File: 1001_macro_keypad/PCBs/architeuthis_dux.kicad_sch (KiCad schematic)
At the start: 32 parts, among them J1 ePaperModule, J2 RotaryModule_01, J3 RotaryModule_02, SW01 MX_SW, SW10 MX_SW, SW11 MX_SW, SW12 MX_SW, SW13 MX_SW, SW14 MX_SW, SW2 MX_SW, SW3 MX_SW, SW4 MX_SW, SW5 MX_SW, SW6 MX_SW, SW7 MX_SW, SW8 MX_SW, SW9 MX_SW, U1 Pico

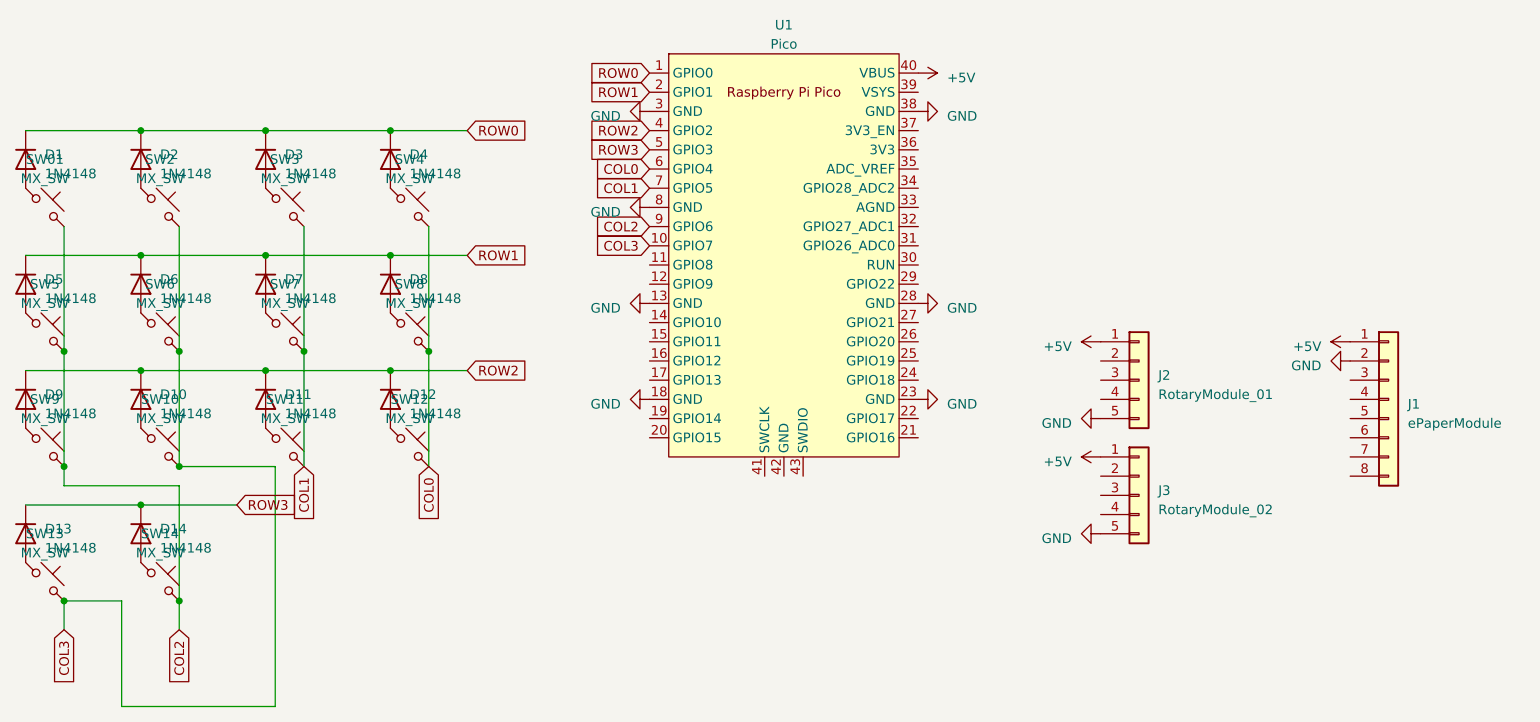
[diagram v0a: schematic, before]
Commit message: 배선작업 거의 완료
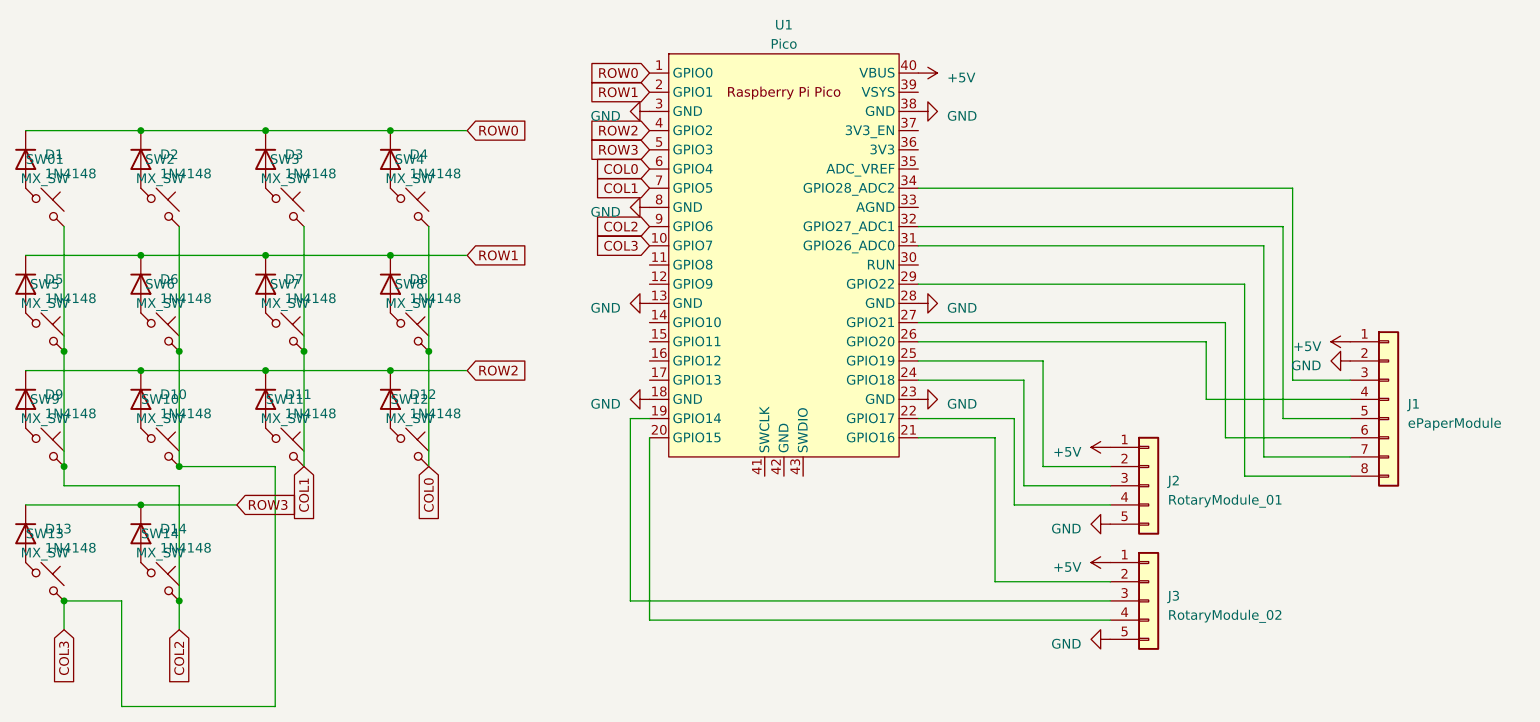
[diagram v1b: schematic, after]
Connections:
- net at J1.3 (D/C): now also U1.34 (GPIO28_ADC2)
- net at J1.4 (CS): now also U1.26 (GPIO20)
- net at J1.5 (SCL): now also U1.32 (GPIO27_ADC1)
- net at J1.6 (SDA): now also U1.27 (GPIO21)
- net at J1.7 (GND): now also U1.31 (GPIO26_ADC0)
- net at J1.8 (VCC): now also U1.29 (GPIO22)
- net at J2.2 (KEY): now also U1.25 (GPIO19)
- net at J2.3 (S2): now also U1.24 (GPIO18)
- net at J2.4 (S1): now also U1.22 (GPIO17)
- net at J3.2 (Pin_2): now also U1.21 (GPIO16)
- net at J3.3 (Pin_3): now also U1.19 (GPIO14)
- net at J3.4 (Pin_4): now also U1.20 (GPIO15)
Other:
- moved on the sheet: J2, J3
